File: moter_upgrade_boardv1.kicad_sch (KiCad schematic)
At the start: 50 parts, among them J1 Conn_01x05_Socket, J2 USB_C_Receptacle_USB2.0_16P, J3 Conn_01x05_Socket, J4 Conn_01x03_Socket, J5 Conn_01x02_Socket, J6 Conn_ST_STDC14, J7 Conn_01x02_Socket, J9 Conn_01x03_Socket, SW1 SW_Wuerth_450301014042, SW3 SW_Push, U1 BD33FC0FP, U3 MCP2562-E-P, U4 BD33FC0FP, U5 TLP785, U6 TLP785, U7 STM32H523CCTx

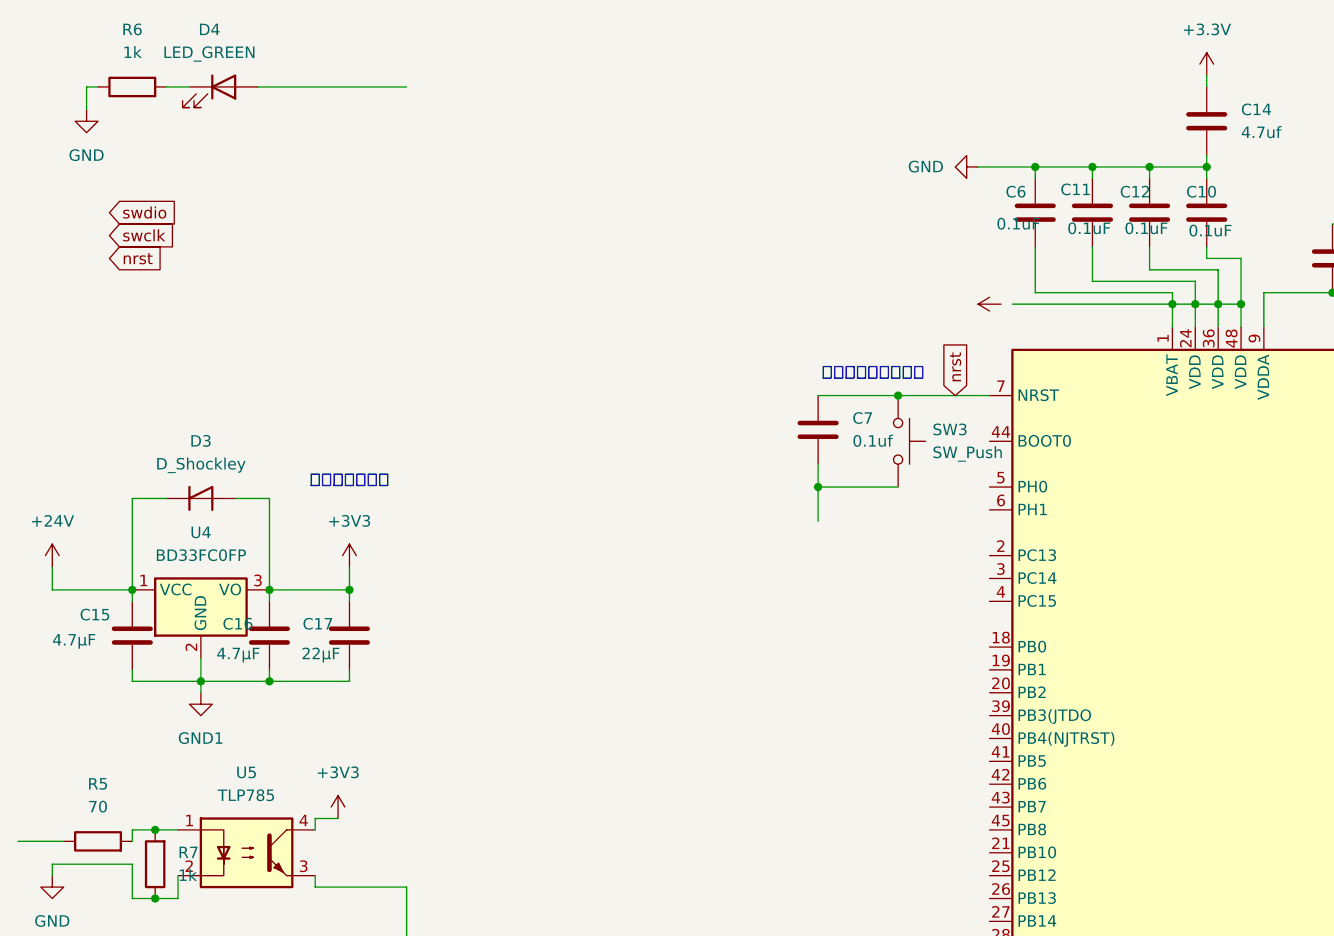
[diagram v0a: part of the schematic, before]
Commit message: a
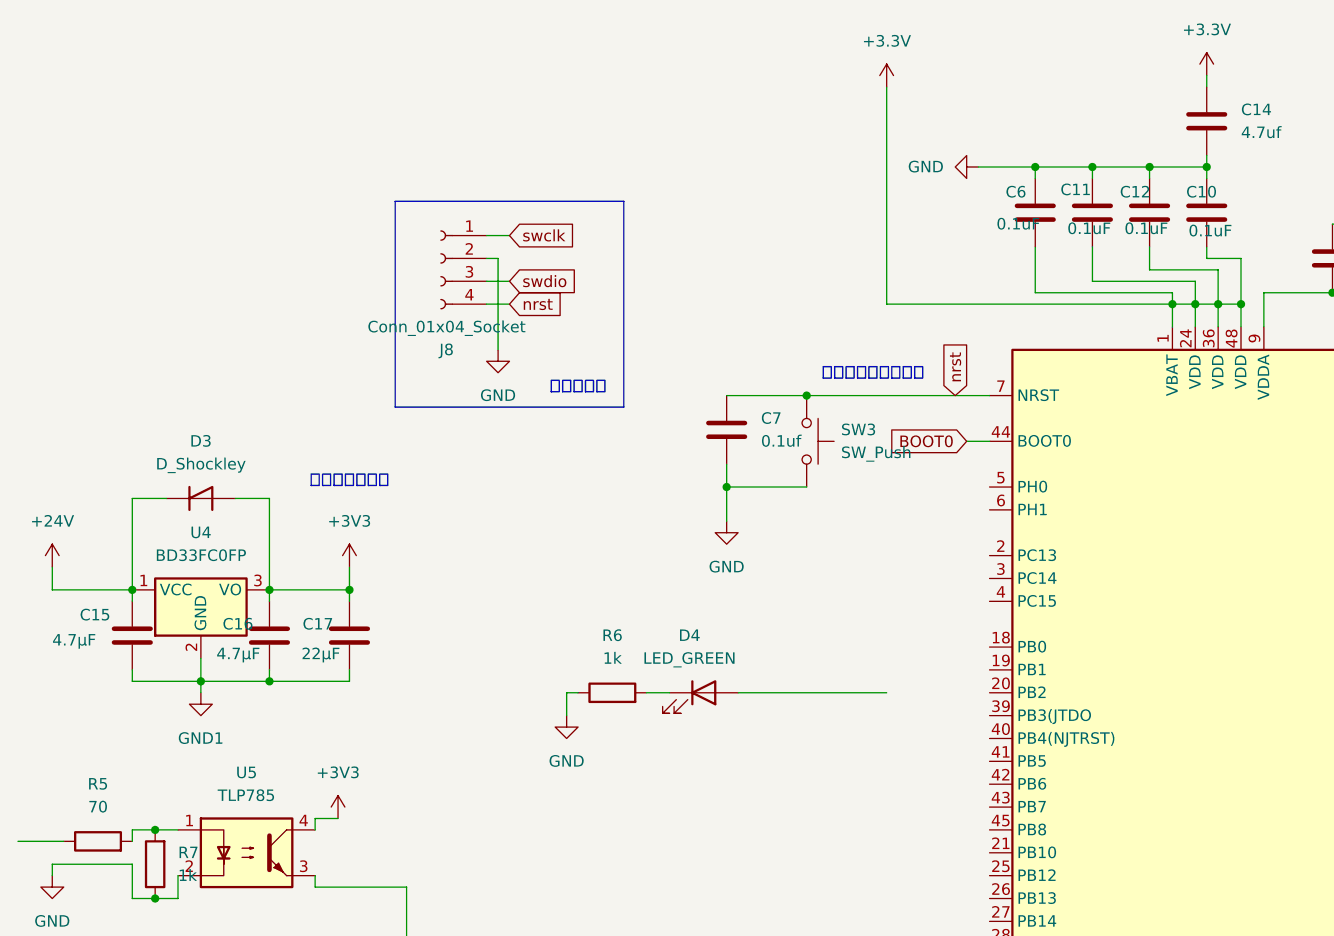
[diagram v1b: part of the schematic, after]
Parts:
- added J8: Conn_01x04_Socket, symbol Connector:Conn_01x04_Socket
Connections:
- net +3.3V: now also C10.1, C11.1, C12.1, C6.1, U7.1 (VBAT), U7.24 (VDD), U7.36 (VDD), U7.48 (VDD)
- net GND: now also C7.2, SW3.2, J8.2 (Pin_2)
- net nrst: now also J8.4 (Pin_4)
- net swclk: now also J8.1 (Pin_1)
- net swdio: now also J8.3 (Pin_3)
- net BOOT0: now reaches U7.44 (BOOT0)
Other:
- note added: "デバッグ用"
- moved on the sheet: C7, D4, R6, SW3

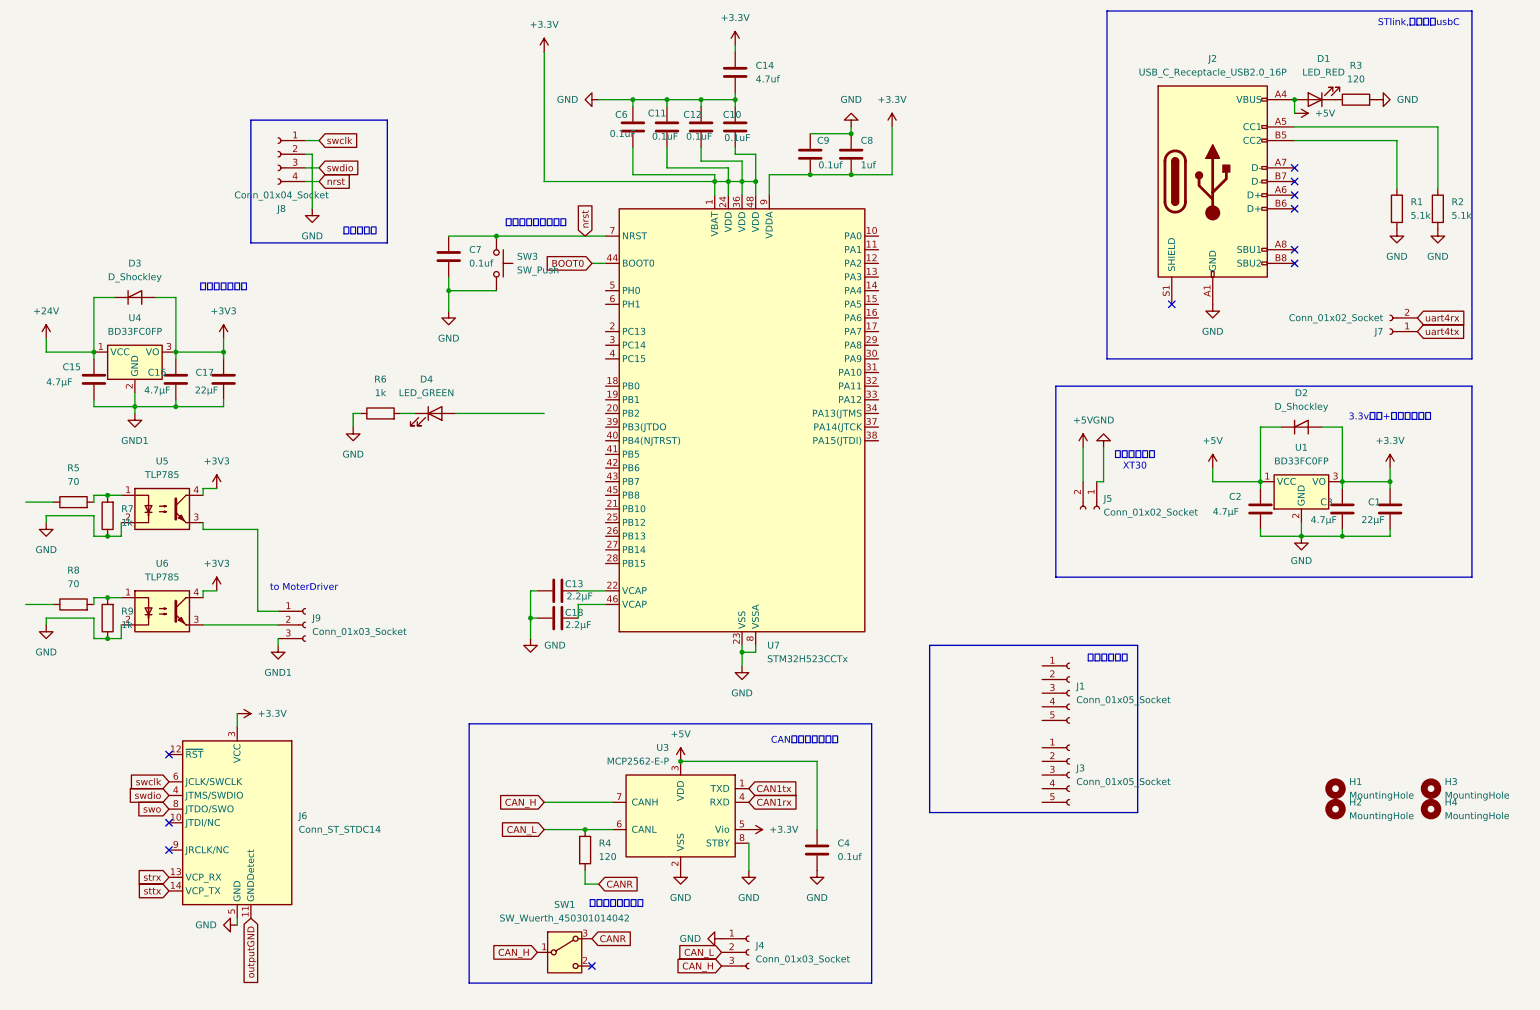
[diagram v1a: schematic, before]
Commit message: 回路図の作図
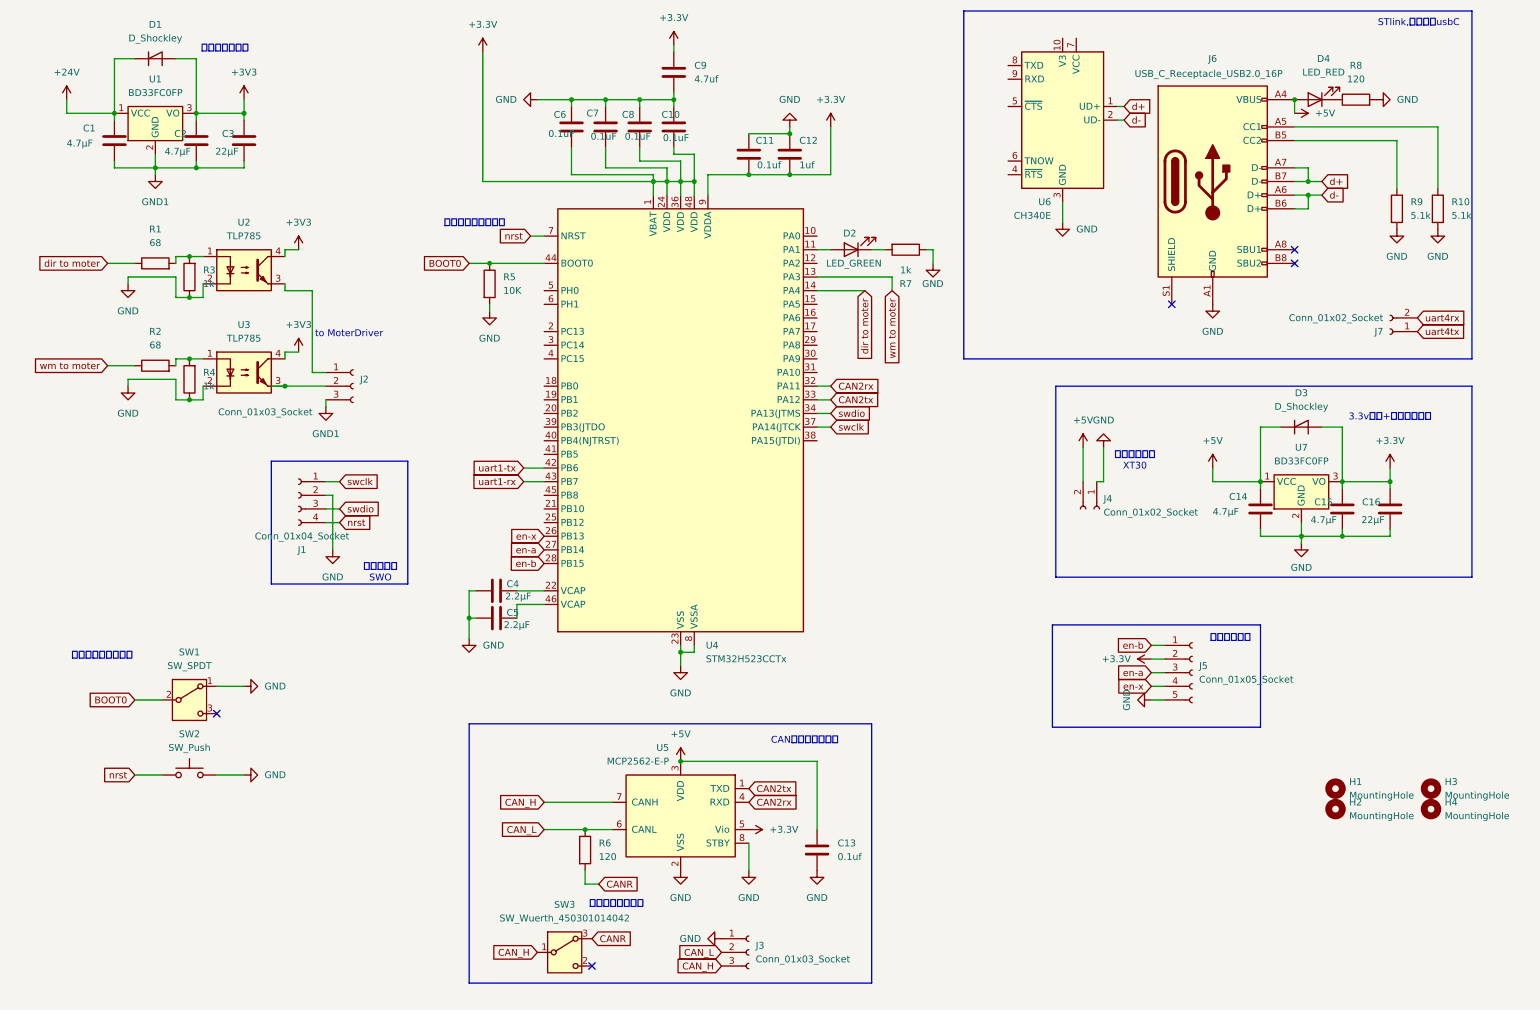
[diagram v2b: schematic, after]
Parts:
- removed C7: 0.1uf, Capacitor_SMD:C_0603_1608Metric_Pad1.08x0.95mm_HandSolder, symbol Device:C
- removed J3: Conn_01x05_Socket, symbol Connector:Conn_01x05_Socket
- removed J6: Conn_ST_STDC14, Connector_PinHeader_1.27mm:PinHeader_2x07_P1.27mm_Vertical, symbol Connector:Conn_ST_STDC14
- removed SW3: SW_Push, Button_Switch_THT:SW_PUSH_6mm, symbol Switch:SW_Push
- added R5: 10K, Resistor_SMD:R_0603_1608Metric_Pad0.98x0.95mm_HandSolder, symbol Device:R
- added SW1: SW_SPDT, Button_Switch_THT:SW_Slide-03_Wuerth-WS-SLTV_10x2.5x6.4_P2.54mm, symbol Switch:SW_SPDT
- added SW2: SW_Push, Button_Switch_THT:SW_PUSH_6mm, symbol Switch:SW_Push
- added U6: CH340E, Package_SO:MSOP-10_3x3mm_P0.5mm, symbol Interface_USB:CH340E
- C10, C6: footprint Capacitor_SMD:C_0402_1005Metric_Pad0.74x0.62mm_HandSolder -> Capacitor_SMD:C_0603_1608Metric_Pad1.08x0.95mm_HandSolder
- C11: renamed from C9; footprint Capacitor_SMD:C_0402_1005Metric_Pad0.74x0.62mm_HandSolder -> Capacitor_SMD:C_0603_1608Metric_Pad1.08x0.95mm_HandSolder
- C5: renamed from C18; footprint Capacitor_SMD:C_0603_1608Metric_Pad1.08x0.95mm_HandSolder -> Capacitor_SMD:C_0805_2012Metric_Pad1.18x1.45mm_HandSolder
- C7: renamed from C11; footprint Capacitor_SMD:C_0402_1005Metric_Pad0.74x0.62mm_HandSolder -> Capacitor_SMD:C_0603_1608Metric_Pad1.08x0.95mm_HandSolder
- C8: renamed from C12; footprint Capacitor_SMD:C_0402_1005Metric_Pad0.74x0.62mm_HandSolder -> Capacitor_SMD:C_0603_1608Metric_Pad1.08x0.95mm_HandSolder
- C9: renamed from C14; footprint Capacitor_SMD:C_0603_1608Metric_Pad1.08x0.95mm_HandSolder -> Capacitor_SMD:C_0805_2012Metric_Pad1.18x1.45mm_HandSolder
- D2: renamed from D4; footprint Diode_SMD:D_0805_2012Metric_Pad1.15x1.40mm_HandSolder -> Capacitor_SMD:C_0603_1608Metric_Pad1.08x0.95mm_HandSolder
- D4: renamed from D1; footprint Diode_SMD:D_0805_2012Metric_Pad1.15x1.40mm_HandSolder -> Capacitor_SMD:C_0603_1608Metric_Pad1.08x0.95mm_HandSolder
- J1: renamed from J8; footprint (none) -> Connector_JST:JST_XH_S4B-XH-A-1_1x04_P2.50mm_Horizontal
- J2: renamed from J9; footprint Connector_JST:JST_XH_S3B-XH-A-1_1x03_P2.50mm_Horizontal -> Connector_PinHeader_2.54mm:PinHeader_1x03_P2.54mm_Vertical
- J5: renamed from J1; footprint (none) -> Connector_JST:JST_XH_S5B-XH-A-1_1x05_P2.50mm_Horizontal
- R1: renamed from R5; value 70 -> 68; footprint Resistor_THT:R_Axial_DIN0207_L6.3mm_D2.5mm_P7.62mm_Horizontal -> Resistor_THT:R_Axial_DIN0207_L6.3mm_D2.5mm_P10.16mm_Horizontal
- R2: renamed from R8; value 70 -> 68; footprint Resistor_THT:R_Axial_DIN0207_L6.3mm_D2.5mm_P7.62mm_Horizontal -> Resistor_THT:R_Axial_DIN0207_L6.3mm_D2.5mm_P10.16mm_Horizontal
- R3: renamed from R7; footprint Resistor_THT:R_Axial_DIN0207_L6.3mm_D2.5mm_P7.62mm_Horizontal -> Resistor_SMD:R_0603_1608Metric_Pad0.98x0.95mm_HandSolder
- R4: renamed from R9; footprint Resistor_THT:R_Axial_DIN0207_L6.3mm_D2.5mm_P7.62mm_Horizontal -> Resistor_SMD:R_0603_1608Metric_Pad0.98x0.95mm_HandSolder
- renumbered C15 to C1, C8 to C12, C4 to C13, C2 to C14, C3 to C15, C1 to C16, C16 to C2, C17 to C3, C13 to C4, D3 to D1, D2 to D3, J4 to J3, J5 to J4, J2 to J6, R2 to R10, R4 to R6, R6 to R7, R3 to R8, R1 to R9, SW1 to SW3, U4 to U1, U5 to U2, U6 to U3, U7 to U4, U3 to U5, U1 to U7
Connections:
- net CAN1rx is gone; now on net CAN2rx: U5.4 (RXD)
- net CAN1tx is gone; now on net CAN2tx: U5.1 (TXD)
- net +3.3V: now also J5.2 (Pin_2)
- net BOOT0: now also R5.1, SW1.2 (B)
- net GND: now also J5.5 (Pin_5), R5.2, SW1.1 (A), SW2.2, U6.3 (GND)
- net nrst: now also SW2.1
- net swclk: now also U4.37 (PA14(JTCK)
- net swdio: now also U4.34 (PA13(JTMS)
- net en-b: now reaches J5.1 (Pin_1)
- net en-b: now also U4.28 (PB15)
- net en-a: now reaches J5.3 (Pin_3)
- net en-a: now also U4.27 (PB14)
- net en-x: now reaches J5.4 (Pin_4)
- net en-x: now also U4.26 (PB13)
- net at U4.11 (PA1): now also D2.2 (A)
- net wm to moter: now reaches U4.13 (PA3)
- net wm to moter: now also R2.1
- net dir to moter: now reaches U4.14 (PA4)
- net dir to moter: now also R1.1
- net CAN2rx: now reaches U4.32 (PA11)
- net CAN2tx: now reaches U4.33 (PA12)
- net uart1-tx: now reaches U4.42 (PB6)
- net uart1-rx: now reaches U4.43 (PB7)
- net d-: now reaches J6.A6 (D+)
- net d-: now also J6.B6 (D+), U6.2 (UD-)
- net d+: now reaches J6.A7 (D-)
- net d+: now also J6.B7 (D-), U6.1 (UD+)
- no-connect marks 11 -> 5
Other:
- note added: "デバッグ用 SWO"
- note removed: "デバッグ用"
- moved on the sheet: C1, C10, C11, C12, C2, C3, C4, C5, C6, C7, C8, C9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
